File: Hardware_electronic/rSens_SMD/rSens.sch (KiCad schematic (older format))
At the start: 20 parts, among them J1 Conn_01x04, J2 Conn_01x04, U2 MCP6244

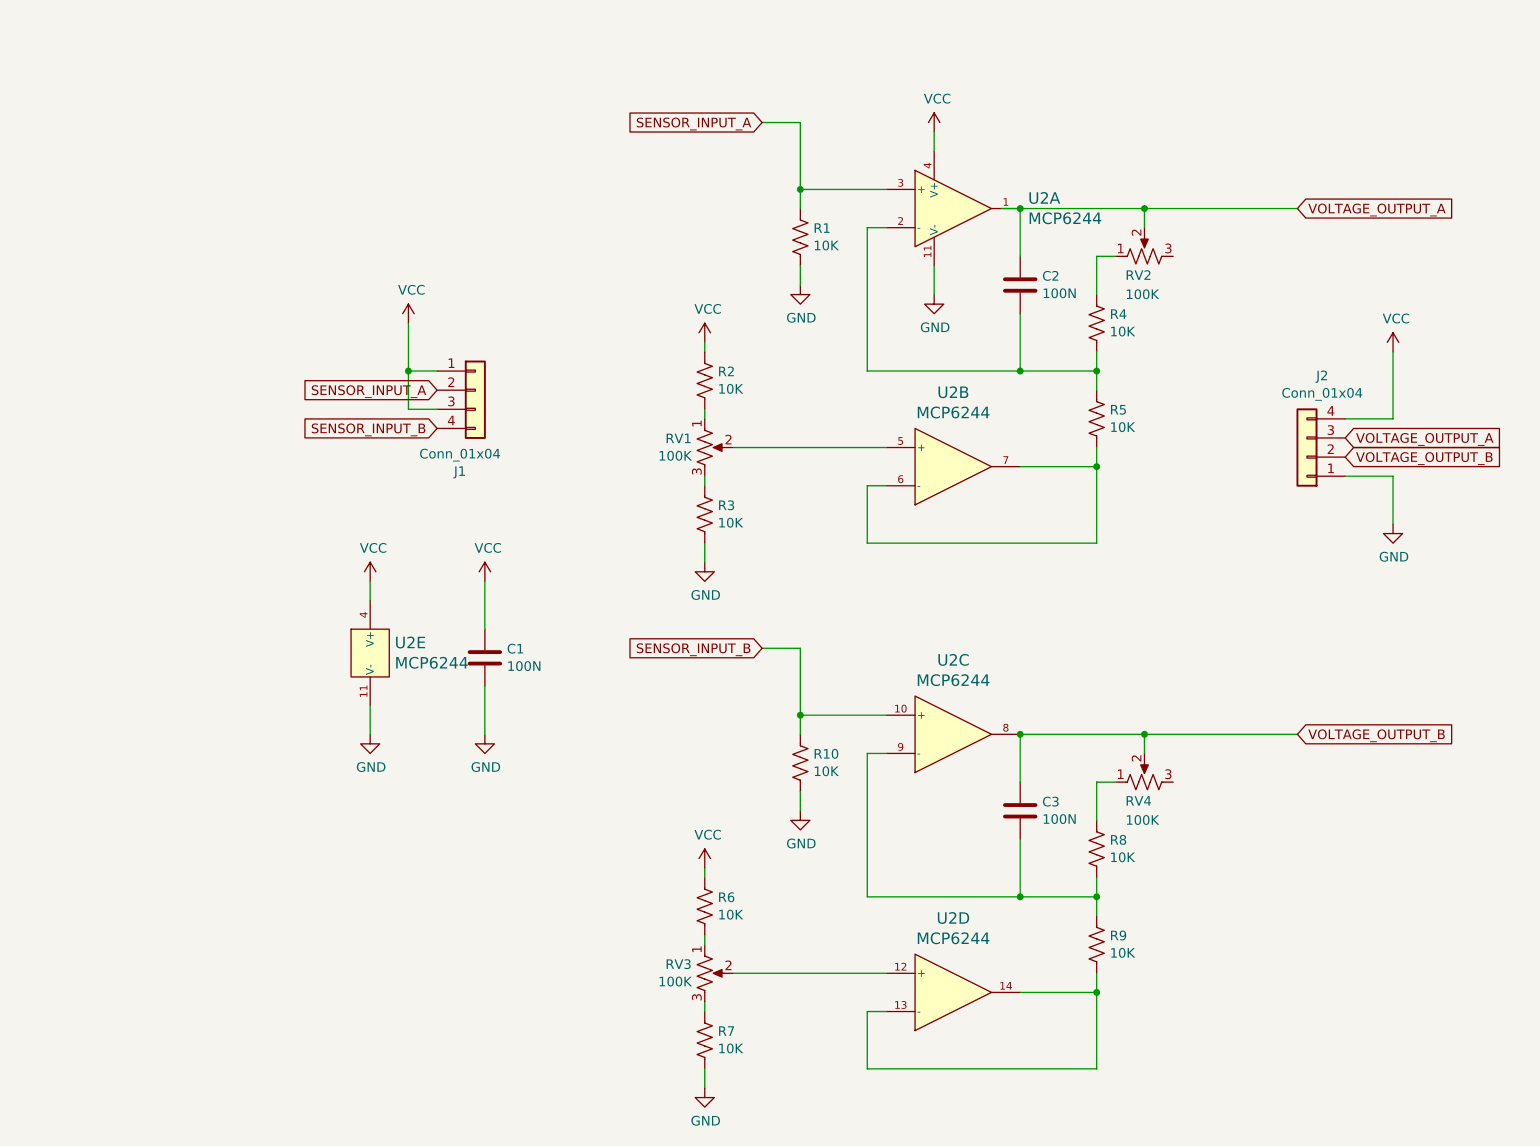
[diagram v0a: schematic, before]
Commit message: CleanUp schematics
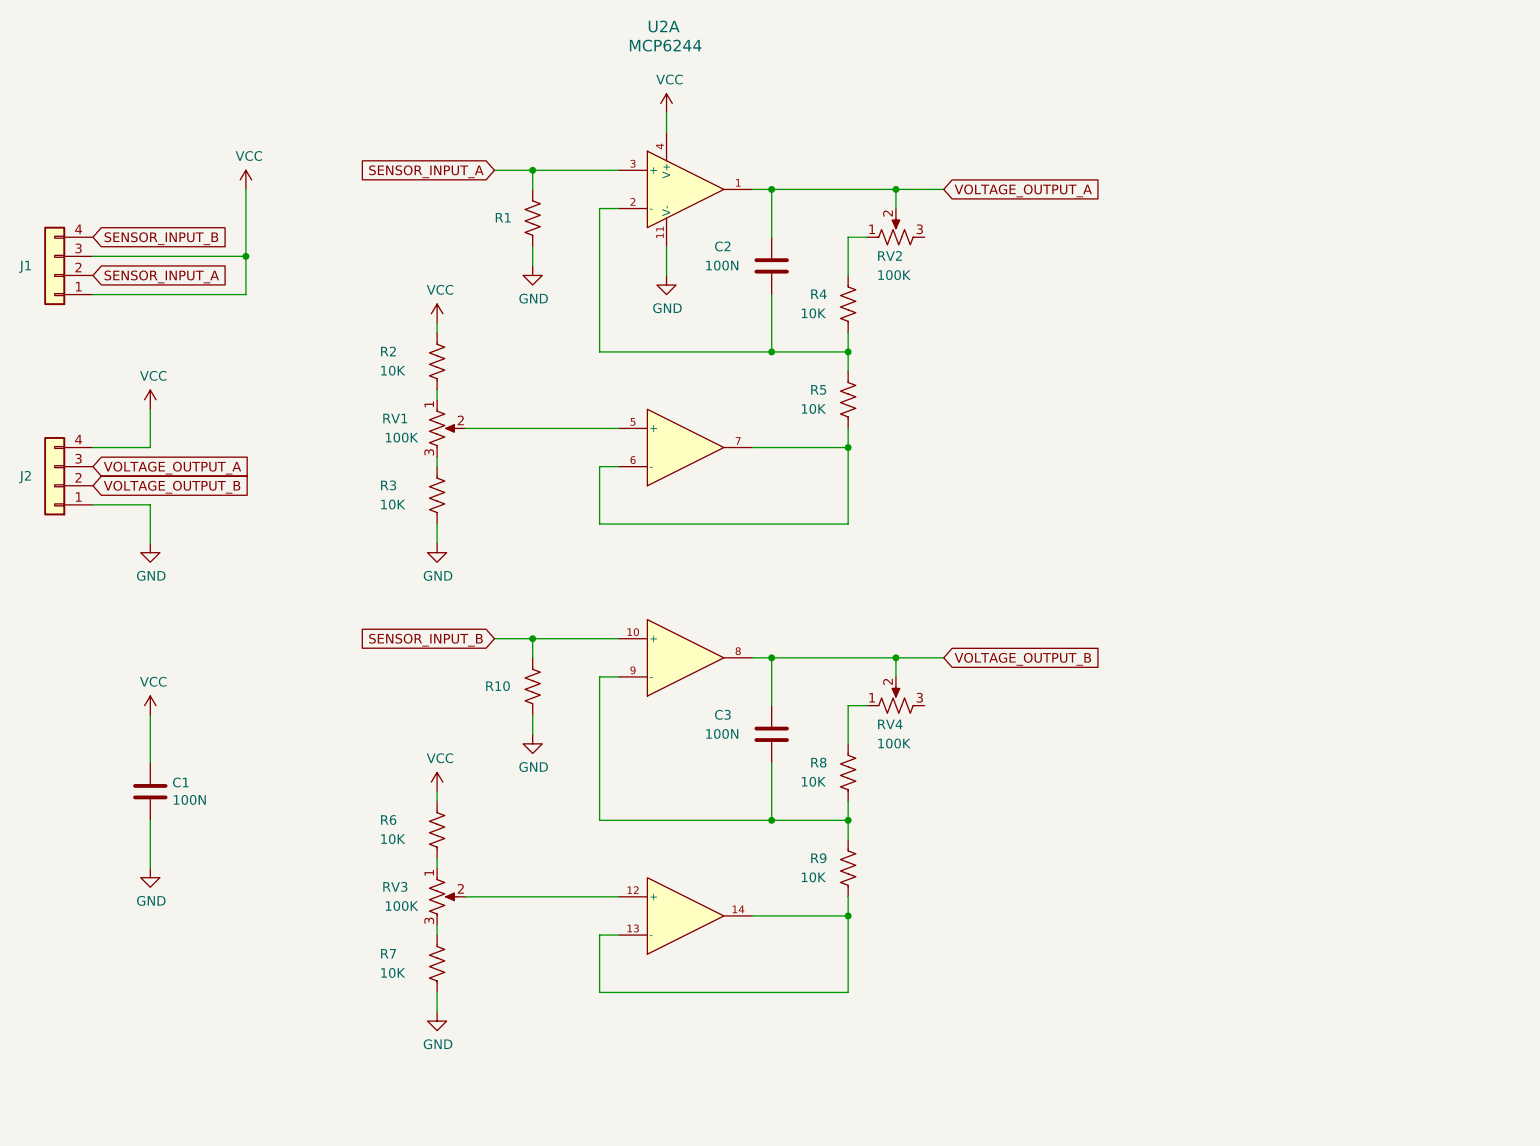
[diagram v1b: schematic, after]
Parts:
- removed unit 5 of U2
- R1, R10: value 10K -> ~
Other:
- moved on the sheet: C1, C2, C3, J1, J2, R1, R10, R2, R3, R4, R5, R6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
